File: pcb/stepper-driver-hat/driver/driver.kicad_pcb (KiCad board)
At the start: 2 copper layers, 70 x 40 mm, 11 parts, among them J1 Conn_01x02, J2 Conn_01x04, J3 Conn_01x04, J4 Conn_01x04, U1 TMC2209_BTT_1.3, U2 TMC2209_BTT_1.3

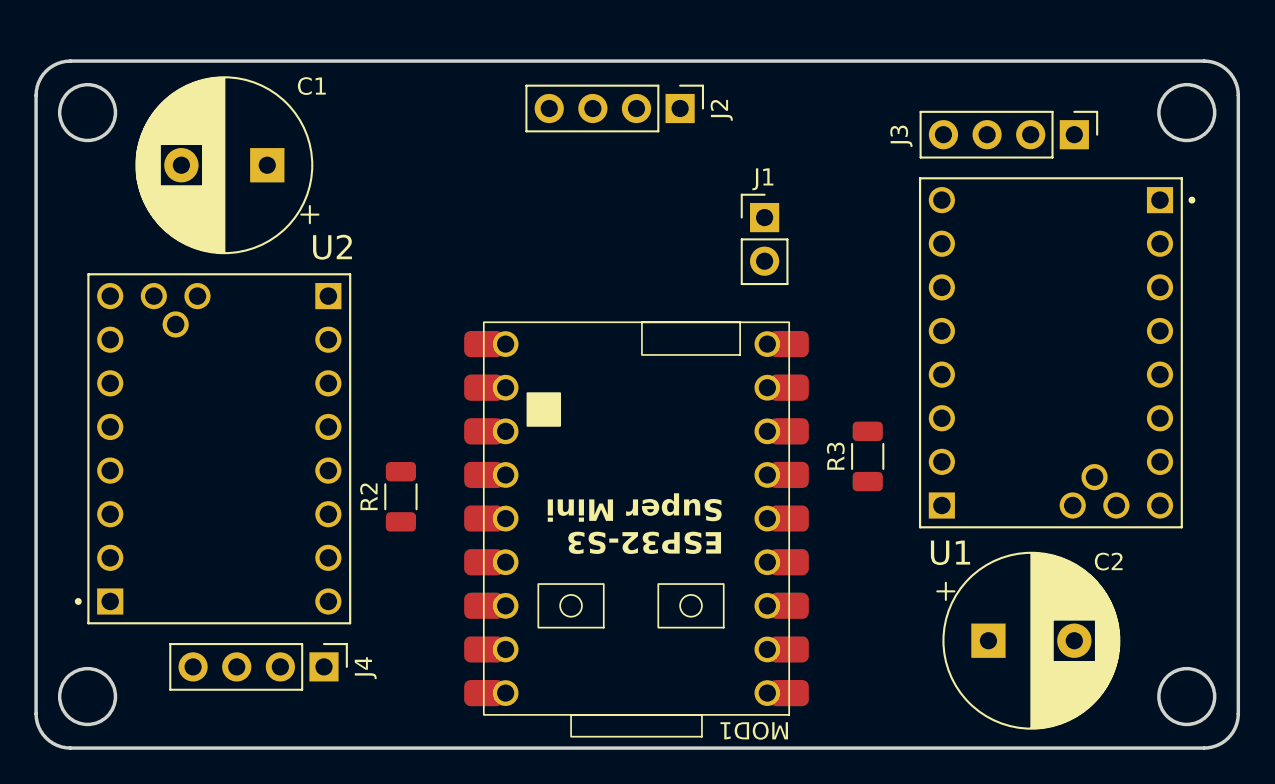
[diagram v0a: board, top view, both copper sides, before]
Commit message: firmeware update
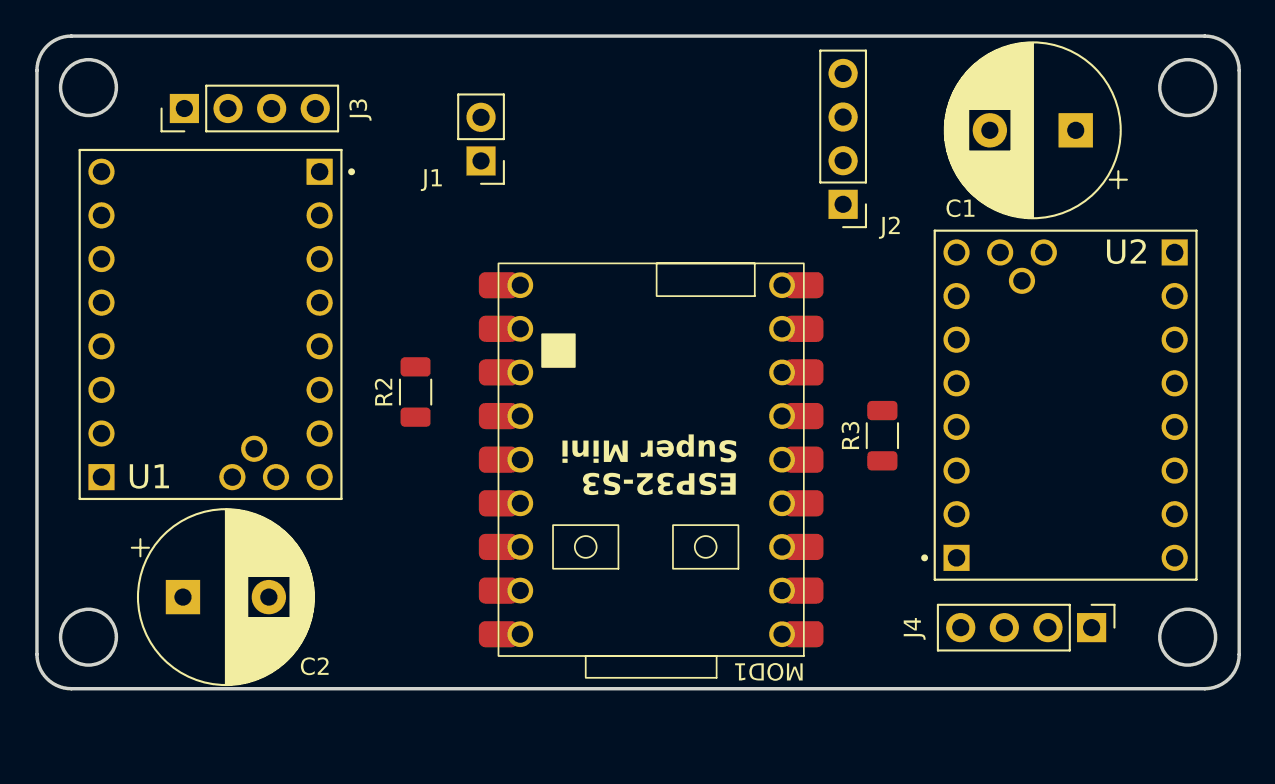
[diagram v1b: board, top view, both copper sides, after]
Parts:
- U1, U2: footprint MotorDrivers:MODULE_TMC2208_SILENTSTEPSTICK -> MotorDrivers:MODULE_TMC2208_TMC2209
- moved J3 51.8 mm to (190.4, 55.3), turned to 90 degrees
- moved U2 49.3 mm to (241.7, 72.6)
- moved U1 49.0 mm to (191.9, 67.9)
- moved C1 47.1 mm to (242.3, 56.6)
- moved C2 47.0 mm to (190.3, 83.8)
- moved J4 44.8 mm to (243.2, 85.6)
- moved J1 16.8 mm to (207.7, 58.4), turned to 180 degrees
- moved J2 11.0 mm to (228.8, 60.9), turned to 180 degrees
- moved R2 6.16 mm to (203.9, 71.8)
- moved MOD1 3.53 mm to (226.5, 85.9)
- moved R3 1.48 mm to (231.1, 74.4)
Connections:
- MOD1 pad 10: DIR_1 -> DIR_0
- MOD1 pad 11: STEP_1 -> STEP_0
- MOD1 pad 12: DIAG_1 -> PDN_0
- MOD1 pad 13: PDN_1 -> Net-(MOD1-GP11)
- MOD1 pad 14: Net-(MOD1-GP12) -> EN_0
- MOD1 pad 15: EN_1 -> DIAG_0
- MOD1 pad 3: DIR_0 -> DIR_1
- MOD1 pad 4: STEP_0 -> STEP_1
- MOD1 pad 5: DIAG_0 -> PDN_1
- MOD1 pad 6: PDN_0 -> Net-(MOD1-GP4)
- MOD1 pad 7: Net-(MOD1-GP5) -> EN_1
- MOD1 pad 8: EN_0 -> DIAG_1
- R2 pad 1: Net-(MOD1-GP12) -> Net-(MOD1-GP11)
- R2 pad 2: PDN_1 -> PDN_0
- R3 pad 1: PDN_0 -> PDN_1
- R3 pad 2: Net-(MOD1-GP5) -> Net-(MOD1-GP4)
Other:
- board size 70 x 40 mm -> 70 x 38 mm
